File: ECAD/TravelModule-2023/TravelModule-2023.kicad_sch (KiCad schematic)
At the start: 7 parts, among them J1 PMW3901, J2 BNO055, U1 Teensy3.2

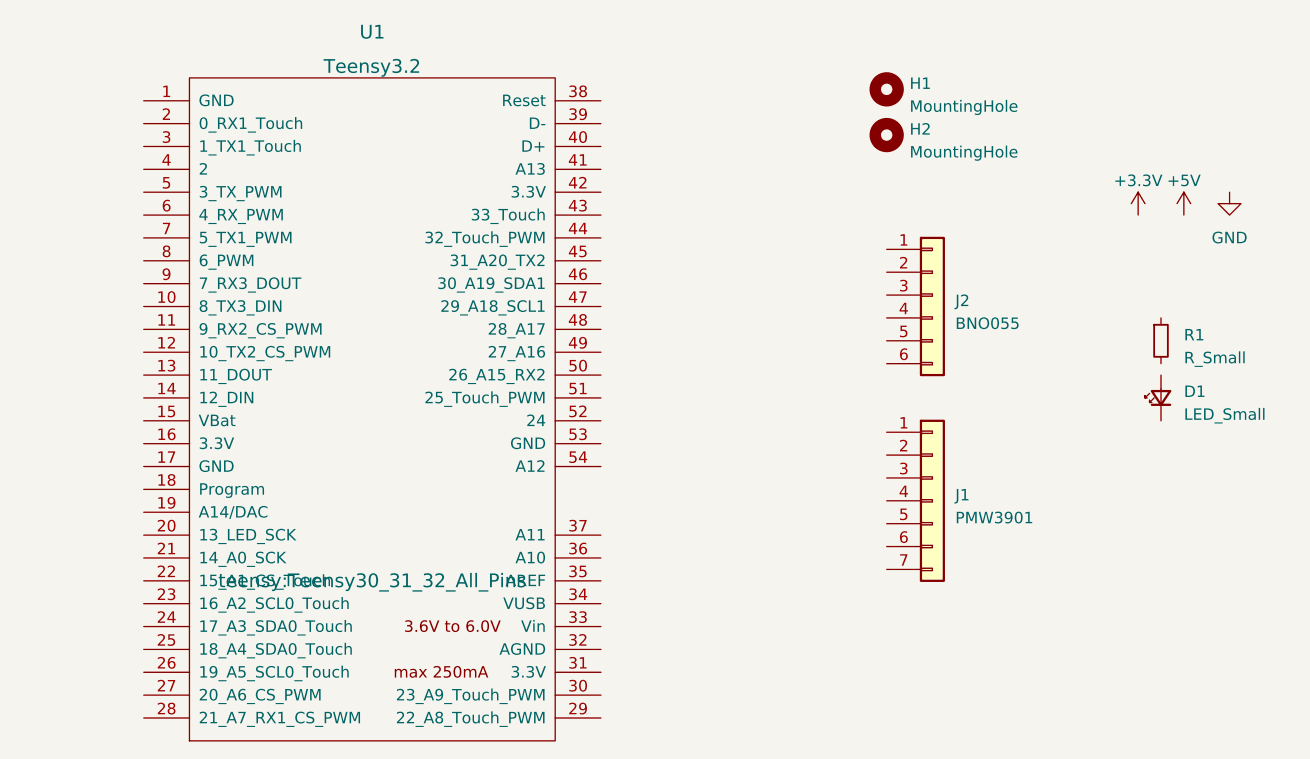
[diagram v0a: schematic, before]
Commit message: Update TravelModule-2023.kicad_sch
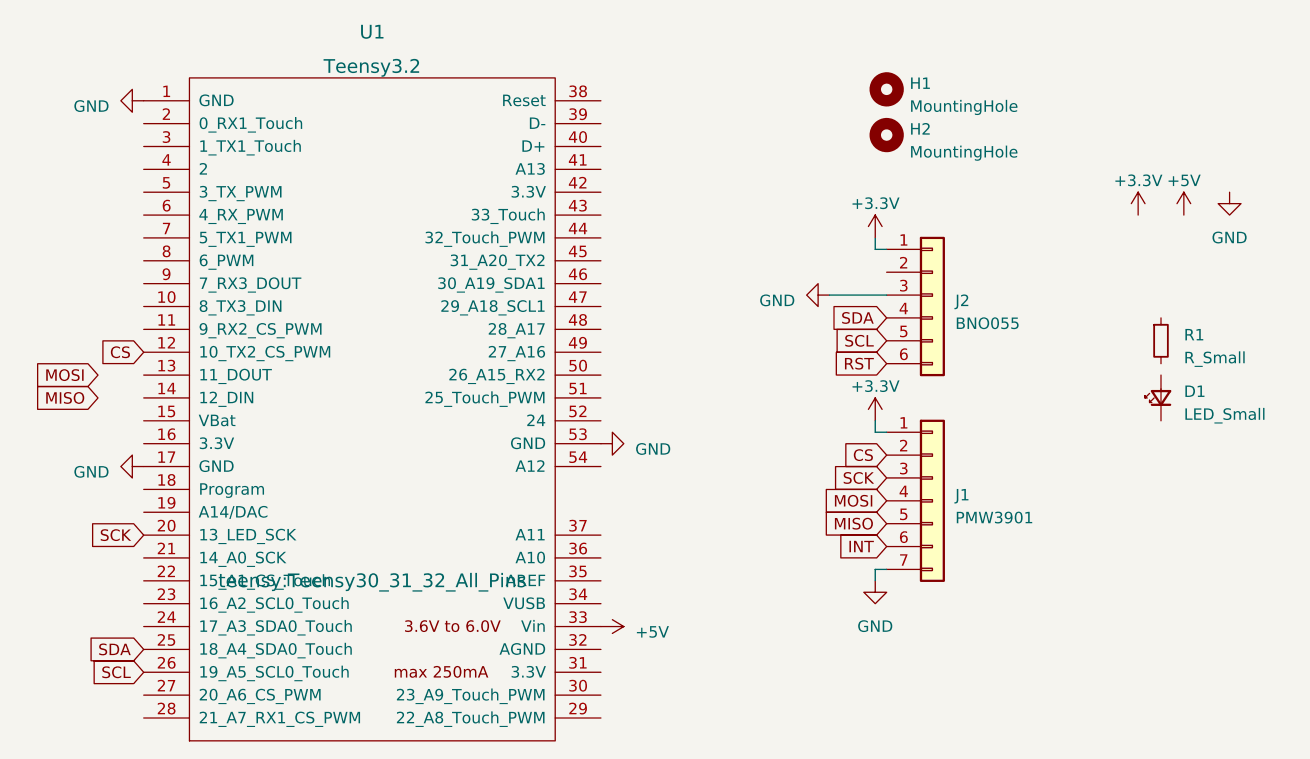
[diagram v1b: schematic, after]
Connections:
- net +3.3V: now also J1.1 (Pin_1), J2.1 (Pin_1)
- net +5V: now also U1.33 (Vin)
- net GND: now also J1.7 (Pin_7), J2.3 (Pin_3), U1.1 (GND), U1.17 (GND), U1.53 (GND)
- net CS: now reaches U1.12 (10_TX2_CS_PWM)
- net CS: now also J1.2 (Pin_2)
- net SCK: now reaches U1.20 (13_LED_SCK)
- net SCK: now also J1.3 (Pin_3)
- net SDA: now reaches U1.25 (18_A4_SDA0_Touch)
- net SDA: now also J2.4 (Pin_4)
- net SCL: now reaches U1.26 (19_A5_SCL0_Touch)
- net SCL: now also J2.5 (Pin_5)
- net RST: now reaches J2.6 (Pin_6)
- net MOSI: now reaches J1.4 (Pin_4)
- net MISO: now reaches J1.5 (Pin_5)
- net INT: now reaches J1.6 (Pin_6)
